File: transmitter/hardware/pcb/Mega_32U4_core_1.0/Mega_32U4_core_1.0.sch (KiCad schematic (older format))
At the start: 37 parts

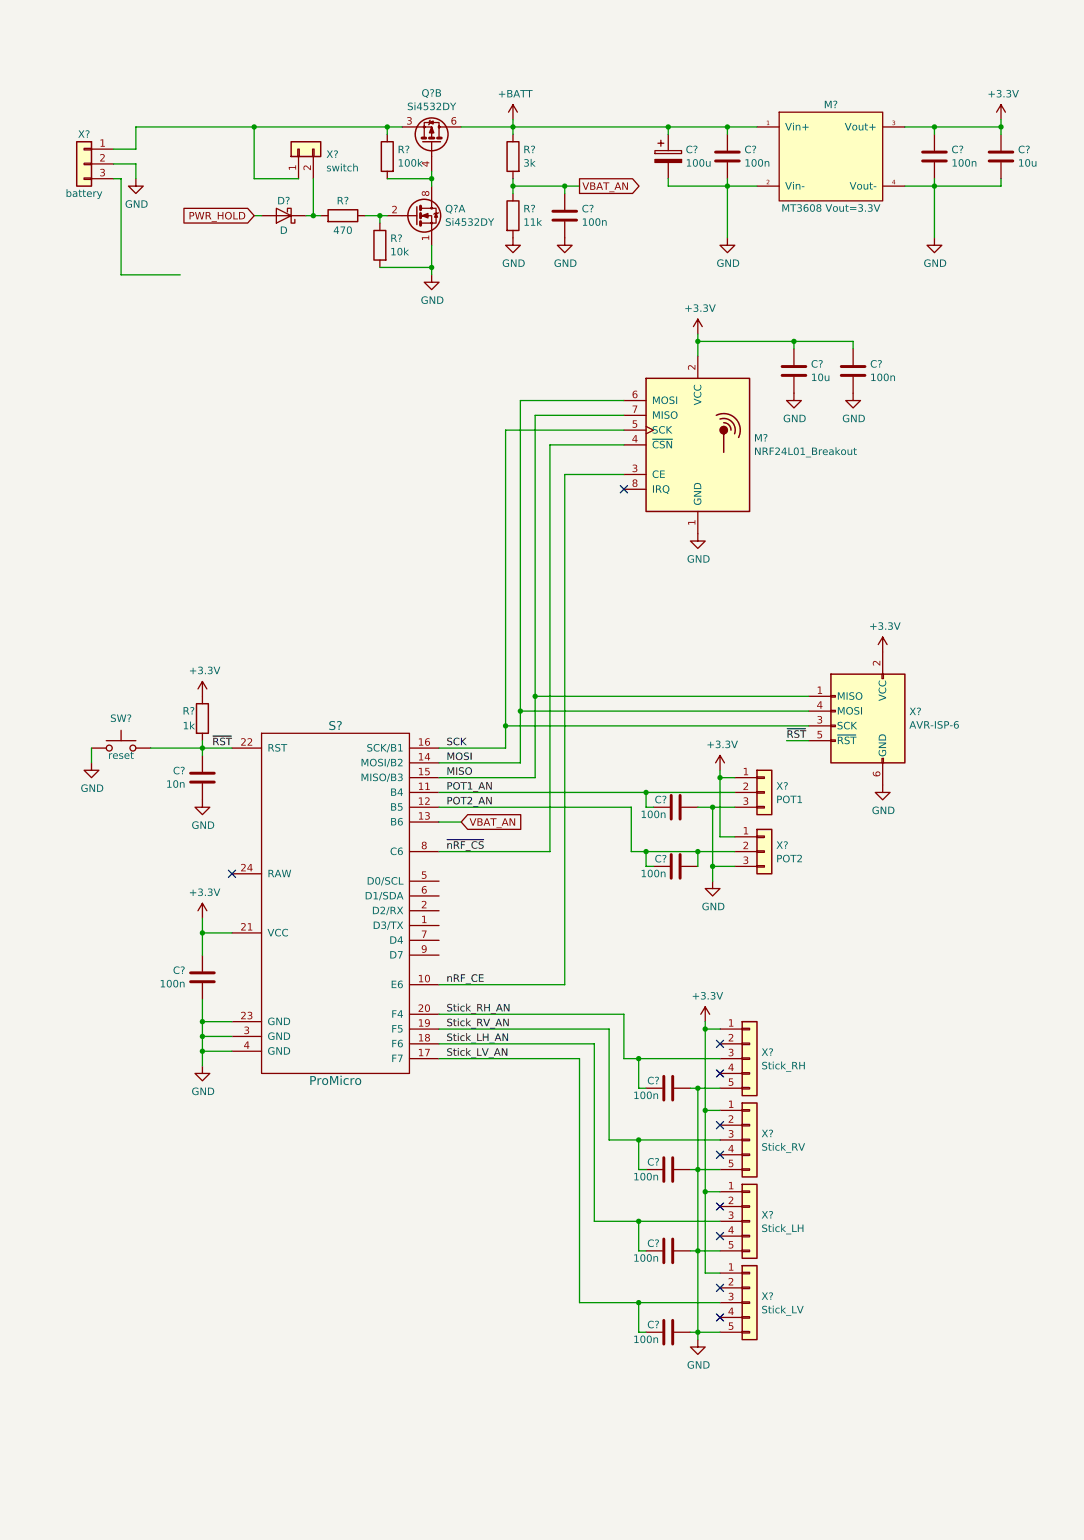
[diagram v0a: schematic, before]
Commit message: WIP
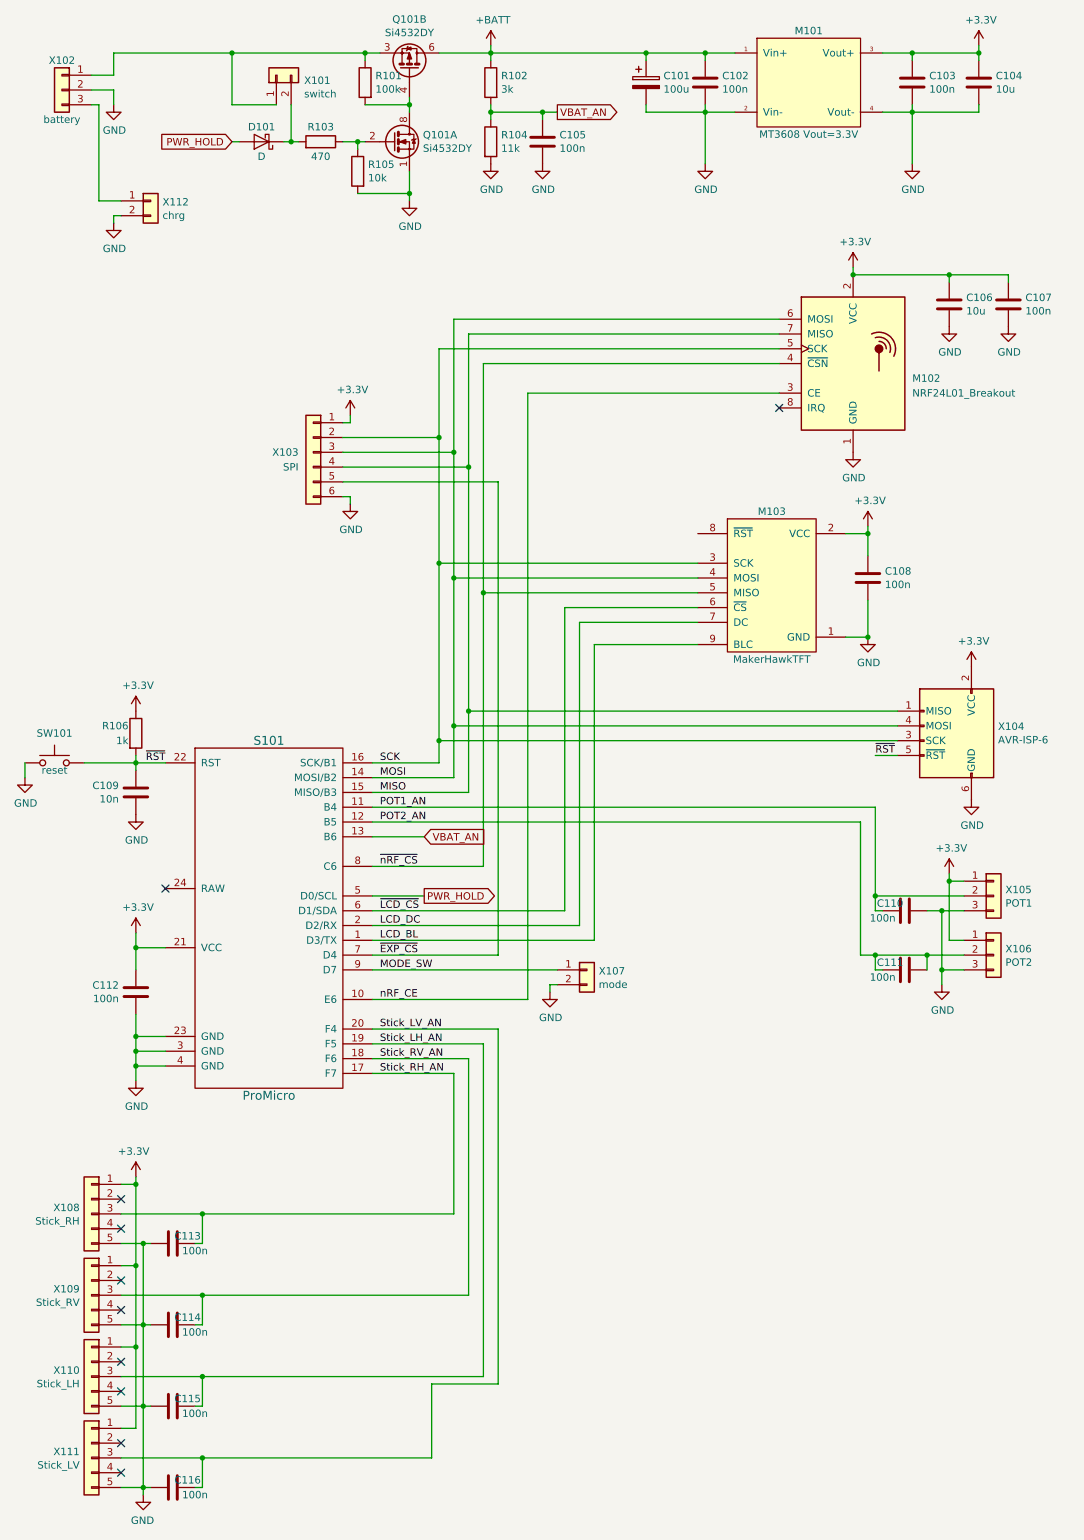
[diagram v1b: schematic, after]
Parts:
- added C108: 100n, Capacitor_SMD:C_0603_1608Metric, symbol Device:C
- added M103: MakerHawkTFT, Connector_PinSocket_2.54mm:PinSocket_1x09_P2.54mm_Vertical, symbol SilentWorks:MakerHawkTFT
- added X103: SPI, Connector_PinSocket_2.54mm:PinSocket_1x06_P2.54mm_Vertical, symbol Connector_Generic:Conn_01x06
- added X107: mode, Connector_PinSocket_2.54mm:PinSocket_1x02_P2.54mm_Vertical, symbol Connector_Generic:Conn_01x02
- added X112: chrg, Connector_PinSocket_2.54mm:PinSocket_1x02_P2.54mm_Vertical, symbol Connector_Generic:Conn_01x02
- C101: renamed from C?; footprint (none) -> Capacitor_SMD:CP_Elec_10x10
- C102, C103, C105, C107, C109, C110, C111, C112, C113, C114, C115, C116: renamed from C?; footprint (none) -> Capacitor_SMD:C_0603_1608Metric
- C104, C106: renamed from C?; footprint (none) -> Capacitor_SMD:C_1206_3216Metric
- D101: renamed from D?; footprint (none) -> Diode_SMD:D_SMA
- M101: renamed from M?; footprint (none) -> SilentWorks:MT3608_module
- R101, R102, R103, R104, R105, R106: renamed from R?; footprint (none) -> Resistor_SMD:R_0603_1608Metric
- S101: renamed from S?; footprint (none) -> SilentWorks:ProMicro
- SW101: renamed from SW?; footprint (none) -> Button_Switch_THT:SW_PUSH_6mm_H4.3mm
- X101: renamed from X?; footprint (none) -> Connector_PinSocket_2.54mm:PinSocket_1x02_P2.54mm_Vertical
- X102: renamed from X?; footprint (none) -> Connector_Molex:Molex_KK-254_AE-6410-03A_1x03_P2.54mm_Vertical
- X104: renamed from X?; footprint (none) -> Connector_IDC:IDC-Header_2x03_P2.54mm_Vertical
- X105, X106: renamed from X?; footprint (none) -> Connector_PinSocket_2.54mm:PinSocket_1x03_P2.54mm_Vertical
- X108, X109, X110, X111: renamed from X?; footprint (none) -> Connector_Molex:Molex_KK-254_AE-6410-05A_1x05_P2.54mm_Vertical
- gave numbers to parts that had none: 2
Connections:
- net +3V3: now also C108.1, M103.2 (VCC), X103.1 (Pin_1)
- net GND: now also C108.2, M103.1 (GND), X103.6 (Pin_6), X107.2 (Pin_2), X112.2 (Pin_2)
- net MISO: now also X103.4 (Pin_4)
- net MOSI: now also M103.4 (MOSI), X103.3 (Pin_3)
- net PWR_HOLD: now also S101.5 (D0/SCL)
- net SCK: now also M103.3 (SCK), X103.2 (Pin_2)
- net Stick_LH_AN: now also S101.19 (F5); no longer S101.18 (F6)
- net Stick_LV_AN: now also S101.20 (F4); no longer S101.17 (F7)
- net Stick_RH_AN: now also S101.17 (F7); no longer S101.20 (F4)
- net Stick_RV_AN: now also S101.18 (F6); no longer S101.19 (F5)
- net ~nRF_CS: now also M103.5 (MISO)
- net LCD_BL: now reaches S101.1 (D3/TX)
- net LCD_BL: now also M103.9 (BLC)
- net LCD_DC: now reaches S101.2 (D2/RX)
- net LCD_DC: now also M103.7 (DC)
- net ~LCD_CS: now reaches S101.6 (D1/SDA)
- net ~LCD_CS: now also M103.6 (~CS)
- net ~EXP_CS: now reaches S101.7 (D4)
- net ~EXP_CS: now also X103.5 (Pin_5)
- net MODE_SW: now reaches S101.9 (D7)
- net MODE_SW: now also X107.1 (Pin_1)
- net at X102.3 (Pin_3): now also X112.1 (Pin_1)
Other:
- moved on the sheet: C101, C102, C103, C104, C105, C106, C107, C109, C110, C111, C112, C113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
